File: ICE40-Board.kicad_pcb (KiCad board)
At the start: 4 copper layers, 134.4 x 58 mm, 82 parts, among them SW1 SW_Push, U1 ADP1712AUJZ-3.3, U10 FT4222HQ, U11 74LS125, U12 74LS126, U2 ADP1712AUJZ-2.5, U3 ADP1712AUJZ-1.2, U4 Barrel_Jack, U5 W25X20CLSNIG, U6 USB_C_Receptacle_USB2.0, U7 ICE40HX4K-TQ144, U8 W25X20CLSNIG, U9 SIT2001BI-S2-33E-25.000000G

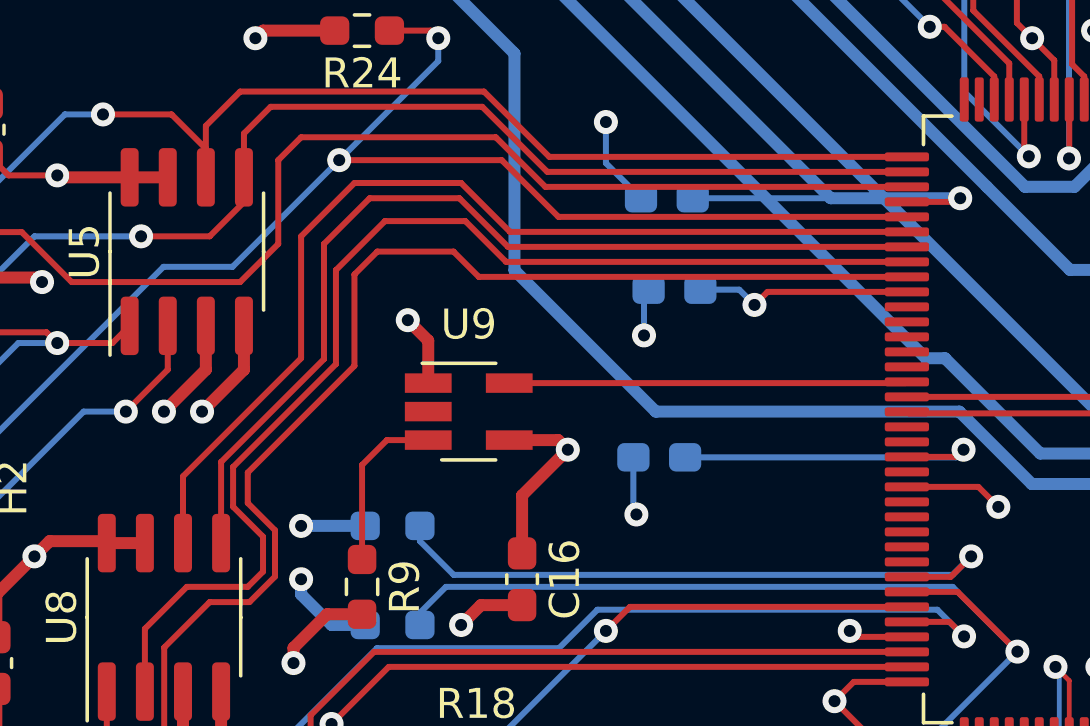
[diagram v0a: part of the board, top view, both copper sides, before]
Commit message: Minor changed
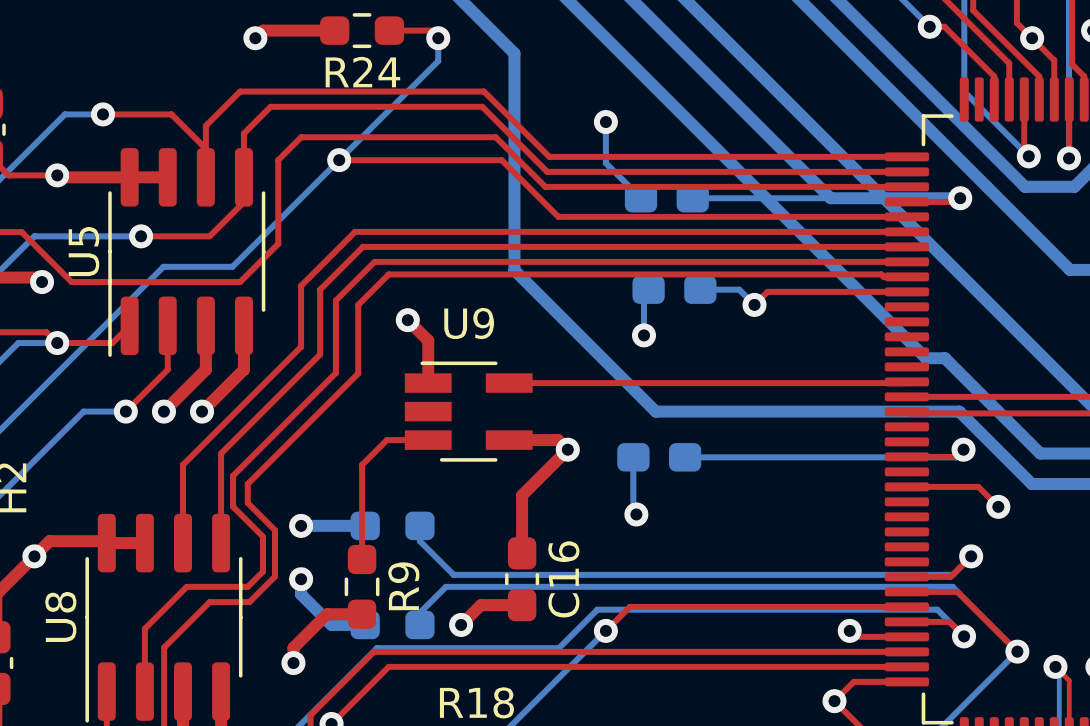
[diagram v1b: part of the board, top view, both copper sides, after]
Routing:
- net Net-(U7-Pad42): track 33.5 -> 31.1 mm
- net Net-(U7-Pad43): track 32.1 -> 30.0 mm
- net Net-(U7-Pad44): track 39.0 -> 37.3 mm
- net Net-(U7-Pad45): track 43.6 -> 42.3 mm
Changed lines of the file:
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@@
   (gr_line (start 22.987 74.676) (end 152.908 74.676) (layer "Edge.Cuts") (width 0.1))
   (gr_arc (start 20.701 18.796) (mid 21.333356 17.269356) (end 22.86 16.637) (layer "Edge.Cuts") (width 0.1))
-  (segment (start 101.9355 40.4675) (end 116.205 40.4675) (width 0.2) (layer "F.Cu") (net 1))
-  (segment (start 98.552 39.624) (end 101.092 39.624) (width 0.2) (layer "F.Cu") (net 1))
-  (segment (start 94.234 46.99) (end 97.79 43.434) (width 0.2) (layer "F.Cu") (net 1))
-  (segment (start 94.291006 51.308) (end 95.14152 50.457486) (width 0.2) (layer "F.Cu") (net 1))
-  (segment (start 89.916 56.896) (end 90.678 56.896) (width 0.2) (layer "F.Cu") (net 1))
-  (segment (start 94.234 48.006) (end 94.234 46.99) (width 0.2) (layer "F.Cu") (net 1))
-  (segment (start 95.14152 48.91352) (end 94.234 48.006) (width 0.2) (layer "F.Cu") (net 1))
-  (segment (start 97.79 40.386) (end 98.552 39.624) (width 0.2) (layer "F.Cu") (net 1))
+  (segment (start 97.917 43.688) (end 97.917 41.402) (width 0.2) (layer "F.Cu") (net 1))
+  (segment (start 90.678 56.896) (end 91.44848 56.12552) (width 0.2) (layer "F.Cu") (net 1))
   (segment (start 92.964 51.308) (end 94.291006 51.308) (width 0.2) (layer "F.Cu") (net 1))
   (segment (start 95.14152 50.457486) (end 95.14152 48.91352) (width 0.2) (layer "F.Cu") (net 1))
+  (segment (start 91.44848 52.82352) (end 92.964 51.308) (width 0.2) (layer "F.Cu") (net 1))
+  (segment (start 89.535 56.515) (end 89.916 56.896) (width 0.2) (layer "F.Cu") (net 1))
+  (segment (start 115.356349 40.386) (end 115.437849 40.4675) (width 0.2) (layer "F.Cu") (net 1))
+  (segment (start 94.234 48.006) (end 94.234 47.371) (width 0.2) (layer "F.Cu") (net 1))
+  (segment (start 97.917 41.402) (end 98.933 40.386) (width 0.2) (layer "F.Cu") (net 1))
+  (segment (start 115.437849 40.4675) (end 116.205 40.4675) (width 0.2) (layer "F.Cu") (net 1))
+  (segment (start 94.291006 51.308) (end 95.14152 50.457486) (width 0.2) (layer "F.Cu") (net 1))
   (segment (start 89.535 54.291) (end 89.535 56.515) (width 0.2) (layer "F.Cu") (net 1))
-  (segment (start 89.535 56.515) (end 89.916 56.896) (width 0.2) (layer "F.Cu") (net 1))
-  (segment (start 90.678 56.896) (end 91.44848 56.12552) (width 0.2) (layer "F.Cu") (net 1))
-  (segment (start 91.44848 52.82352) (end 92.964 51.308) (width 0.2) (layer "F.Cu") (net 1))
+  (segment (start 98.933 40.386) (end 115.356349 40.386) (width 0.2) (layer "F.Cu") (net 1))
+  (segment (start 94.234 47.371) (end 97.917 43.688) (width 0.2) (layer "F.Cu") (net 1))
   (segment (start 91.44848 56.12552) (end 91.44848 52.82352) (width 0.2) (layer "F.Cu") (net 1))
-  (segment (start 97.79 43.434) (end 97.79 40.386) (width 0.2) (layer "F.Cu") (net 1))
-  (segment (start 101.092 39.624) (end 101.9355 40.4675) (width 0.2) (layer "F.Cu") (net 1))
-  (segment (start 97.17352 40.24048) (end 98.806 38.608) (width 0.2) (layer "F.Cu") (net 2))
-  (segment (start 102.845488 39.9675) (end 116.205 39.9675) (width 0.2) (layer "F.Cu") (net 2))
+  (segment (start 89.916 56.896) (end 90.678 56.896) (width 0.2) (layer "F.Cu") (net 1))
+  (segment (start 95.14152 48.91352) (end 94.234 48.006) (width 0.2) (layer "F.Cu") (net 1))
+  (segment (start 97.17352 41.25648) (end 98.4625 39.9675) (width 0.2) (layer "F.Cu") (net 2))
+  (segment (start 90.805 54.291) (end 90.805 52.197) (width 0.2) (layer "F.Cu") (net 2))
   (segment (start 94.742 50.292) (end 94.742 49.127283) (width 0.2) (layer "F.Cu") (net 2))
-  (segment (start 101.485988 38.608) (end 102.845488 39.9675) (width 0.2) (layer "F.Cu") (net 2))
-  (segment (start 93.74452 48.129803) (end 93.74452 46.802989) (width 0.2) (layer "F.Cu") (net 2))
-  (segment (start 98.806 38.608) (end 101.485988 38.608) (width 0.2) (layer "F.Cu") (net 2))
   (segment (start 94.234 50.8) (end 94.742 50.292) (width 0.2) (layer "F.Cu") (net 2))
-  (segment (start 93.74452 46.802989) (end 97.17352 43.373989) (width 0.2) (layer "F.Cu") (net 2))
+  (segment (start 93.74452 47.09848) (end 97.17352 43.66948) (width 0.2) (layer "F.Cu") (net 2))
+  (segment (start 90.805 52.197) (end 92.202 50.8) (width 0.2) (layer "F.Cu") (net 2))
+  (segment (start 93.74452 48.129803) (end 93.74452 47.09848) (width 0.2) (layer "F.Cu") (net 2))
+  (segment (start 92.202 50.8) (end 94.234 50.8) (width 0.2) (layer "F.Cu") (net 2))
+  (segment (start 98.4625 39.9675) (end 116.205 39.9675) (width 0.2) (layer "F.Cu") (net 2))
+  (segment (start 97.17352 43.66948) (end 97.17352 41.25648) (width 0.2) (layer "F.Cu") (net 2))
   (segment (start 94.742 49.127283) (end 93.74452 48.129803) (width 0.2) (layer "F.Cu") (net 2))
-  (segment (start 90.805 54.291) (end 90.805 52.197) (width 0.2) (layer "F.Cu") (net 2))
-  (segment (start 90.805 52.197) (end 92.202 50.8) (width 0.2) (layer "F.Cu") (net 2))
-  (segment (start 92.202 50.8) (end 94.234 50.8) (width 0.2) (layer "F.Cu") (net 2))
-  (segment (start 97.17352 43.373989) (end 97.17352 40.24048) (width 0.2) (layer "F.Cu") (net 2))
   (segment (start 102.7665 56.134) (end 104.648 56.134) (width 0.4) (layer "F.Cu") (net 3))
   (segment (start 126.1175 58.2865) (end 126.1175 55.88) (width 0.2) (layer "F.Cu") (net 3))
@@
   (segment (start 107.442 42.418) (end 107.442 41.0475) (width 0.2) (layer "B.Cu") (net 4))
   (segment (start 107.188 48.387) (end 107.0875 48.2865) (width 0.2) (layer "B.Cu") (net 4))
-  (segment (start 101.288994 37.846) (end 102.910494 39.4675) (width 0.2) (layer "F.Cu") (net 5))
-  (segment (start 98.298 37.846) (end 101.288994 37.846) (width 0.2) (layer "F.Cu") (net 5))
-  (segment (start 96.774 39.37) (end 98.298 37.846) (width 0.2) (layer "F.Cu") (net 5))
-  (segment (start 93.345 46.637503) (end 96.774 43.208503) (width 0.2) (layer "F.Cu") (net 5))
-  (segment (start 102.910494 39.4675) (end 116.205 39.4675) (width 0.2) (layer "F.Cu") (net 5))
-  (segment (start 93.345 49.341) (end 93.345 46.637503) (width 0.2) (layer "F.Cu") (net 5))
-  (segment (start 96.774 43.208503) (end 96.774 39.37) (width 0.2) (layer "F.Cu") (net 5))
-  (segment (start 101.346 37.338) (end 102.9755 38.9675) (width 0.2) (layer "F.Cu") (net 6))
-  (segment (start 92.075 47.117) (end 96.012 43.18) (width 0.2) (layer "F.Cu") (net 6))
-  (segment (start 102.9755 38.9675) (end 116.205 38.9675) (width 0.2) (layer "F.Cu") (net 6))
-  (segment (start 96.012 43.18) (end 96.012 39.116) (width 0.2) (layer "F.Cu") (net 6))
-  (segment (start 92.075 49.341) (end 92.075 47.117) (width 0.2) (layer "F.Cu") (net 6))
-  (segment (start 96.012 39.116) (end 97.79 37.338) (width 0.2) (layer "F.Cu") (net 6))
-  (segment (start 97.79 37.338) (end 101.346 37.338) (width 0.2) (layer "F.Cu") (net 6))
+  (segment (start 93.345 46.355) (end 96.647 43.053) (width 0.2) (layer "F.Cu") (net 5))
+  (segment (start 96.647 43.053) (end 96.647 40.894) (width 0.2) (layer "F.Cu") (net 5))
+  (segment (start 93.345 49.341) (end 93.345 46.355) (width 0.2) (layer "F.Cu") (net 5))
+  (segment (start 96.647 40.894) (end 98.0735 39.4675) (width 0.2) (layer "F.Cu") (net 5))
+  (segment (start 98.0735 39.4675) (end 116.205 39.4675) (width 0.2) (layer "F.Cu") (net 5))
+  (segment (start 92.075 46.736) (end 96.012 42.799) (width 0.2) (layer "F.Cu") (net 6))
+  (segment (start 96.012 42.799) (end 96.012 40.767) (width 0.2) (layer "F.Cu") (net 6))
+  (segment (start 92.075 49.341) (end 92.075 46.736) (width 0.2) (layer "F.Cu") (net 6))
+  (segment (start 96.012 40.767) (end 97.8115 38.9675) (width 0.2) (layer "F.Cu") (net 6))
+  (segment (start 97.8115 38.9675) (end 116.205 38.9675) (width 0.2) (layer "F.Cu") (net 6))
   (segment (start 97.282 36.576) (end 102.698982 36.576) (width 0.2) (layer "F.Cu") (net 7))
   (segment (start 102.698982 36.576) (end 104.590482 38.4675) (width 0.2) (layer "F.Cu") (net 7))
